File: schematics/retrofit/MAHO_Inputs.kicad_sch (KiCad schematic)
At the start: 3 parts, among them U401 7i97-TB5-OUTPUTS-A, U402 7i97-TB5-OUTPUTS-B

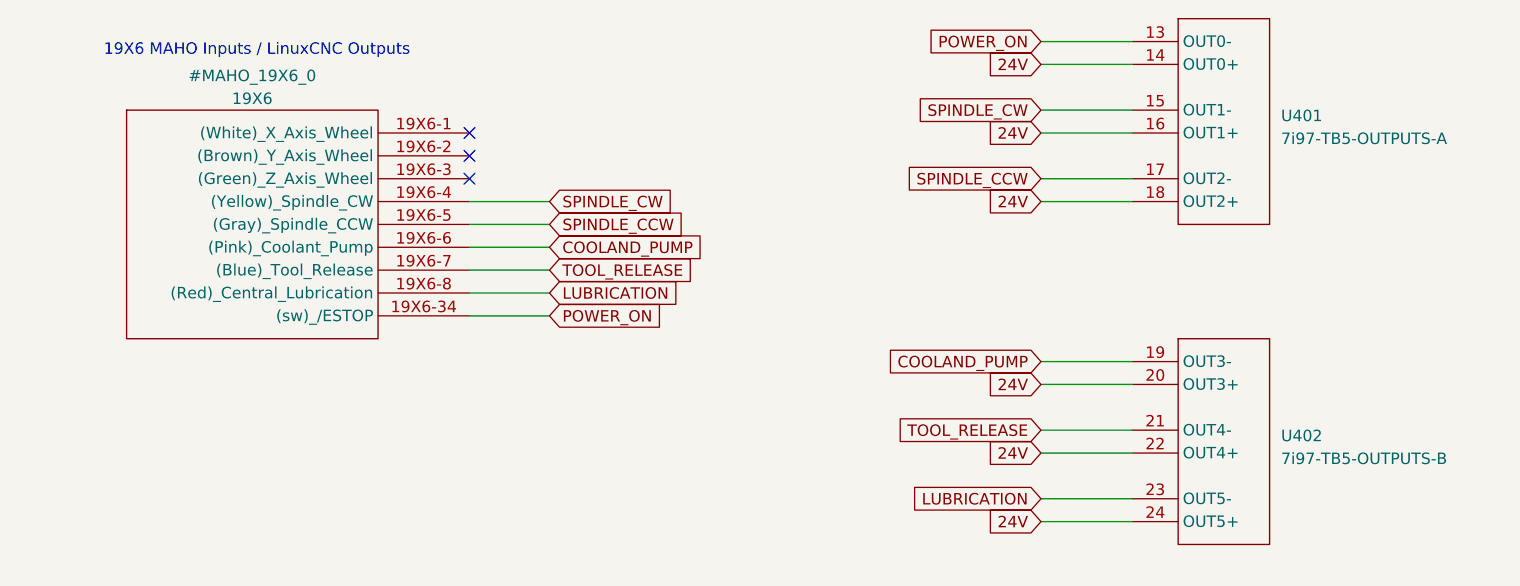
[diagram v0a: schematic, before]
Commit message: schematics
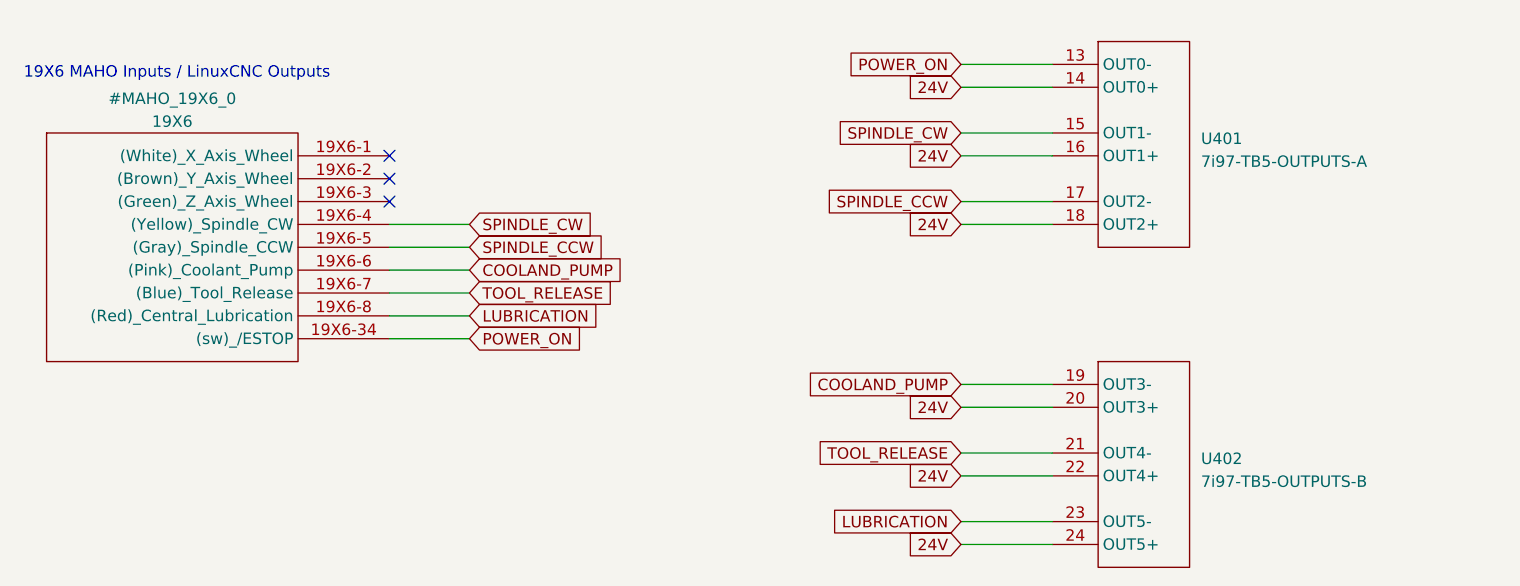
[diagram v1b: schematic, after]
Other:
- moved on the sheet: U401, U402
